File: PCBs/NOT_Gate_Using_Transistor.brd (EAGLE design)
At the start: 23 x 30 mm, 8 parts, among them T1 BC547

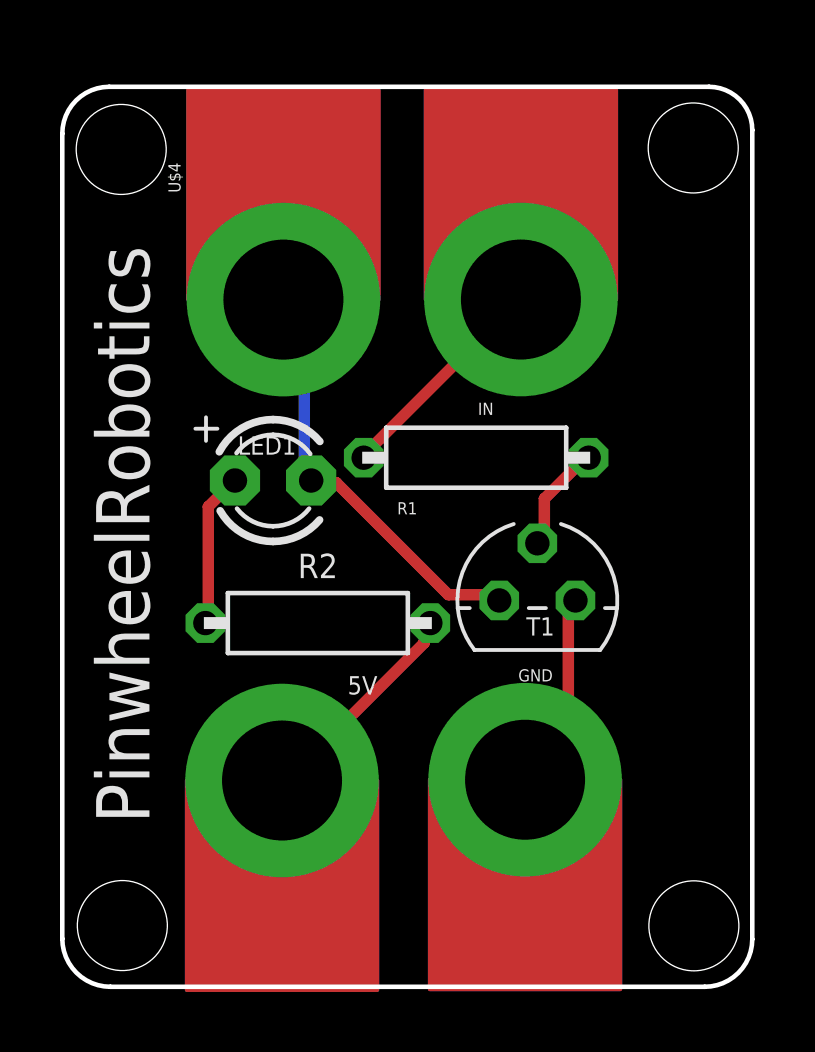
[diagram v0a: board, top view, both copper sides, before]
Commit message: New Update
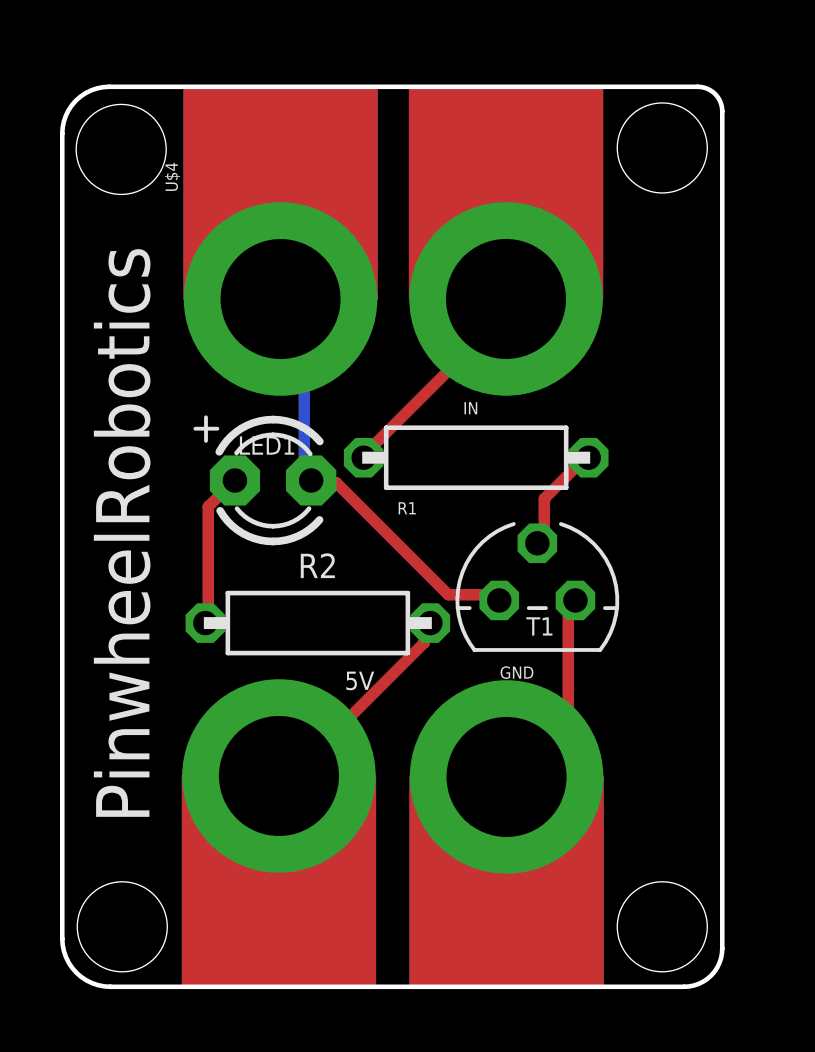
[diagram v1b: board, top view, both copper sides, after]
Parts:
- moved GND 0.62 mm to (11.8, 6.99)
- moved IN 0.50 mm to (11.8, 22.9)
- moved 5V 0.18 mm to (4.22, 7.03)
- moved U$4 0.10 mm to (4.28, 22.9)
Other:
- board size 23 x 30 mm -> 22 x 30 mm
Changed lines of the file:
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@@
 <plain>
 <hole x="-1.036" y="27.912" drill="3"/>
-<hole x="18.031" y="27.961" drill="3"/>
-<hole x="-0.998" y="2.041" drill="3"/>
-<hole x="18.053" y="2.032" drill="3"/>
-<wire x1="-1.3943875" y1="0" x2="18.413571875" y2="0" width="0.1524" layer="20"/>
-<wire x1="18.413571875" y1="0" x2="20" y2="1.586428125" width="0.1524" layer="20" curve="90"/>
-<wire x1="20" y1="1.586428125" x2="20" y2="28.5579125" width="0.1524" layer="20"/>
-<wire x1="20" y1="28.5579125" x2="18.5579125" y2="30" width="0.1524" layer="20" curve="90"/>
-<wire x1="18.5579125" y1="30" x2="-1.437390625" y2="30" width="0.1524" layer="20"/>
+<hole x="17" y="27.961" drill="3"/>
+<hole x="-1" y="2" drill="3"/>
+<hole x="17" y="2" drill="3"/>
+<wire x1="-1.3943875" y1="0" x2="17.7262875" y2="0" width="0.1524" layer="20"/>
+<wire x1="17.7262875" y1="0" x2="19" y2="1.2737125" width="0.1524" layer="20" curve="90"/>
+<wire x1="19" y1="1.2737125" x2="19" y2="29.182434375" width="0.1524" layer="20"/>
+<wire x1="19" y1="29.182434375" x2="18.182434375" y2="30" width="0.1524" layer="20" curve="90"/>
+<wire x1="18.182434375" y1="30" x2="-1.437390625" y2="30" width="0.1524" layer="20"/>
 <wire x1="-1.437390625" y1="30" x2="-3" y2="28.437390625" width="0.1524" layer="20" curve="90"/>
 <wire x1="-3" y1="28.437390625" x2="-3" y2="1.6056125" width="0.1524" layer="20"/>
@@
 </autorouter>
 <elements>
-<element name="5V" library="microbit" package="MICROBIT_PAD" value="MICROBIT_PAD" x="4.325" y="6.876" smashed="yes">
-<attribute name="NAME" x="6.512" y="9.745" size="0.6096" layer="21" font="vector"/>
-</element>
-<element name="GND" library="microbit" package="MICROBIT_PAD" value="MICROBIT_PAD" x="12.426" y="6.902" smashed="yes">
-<attribute name="NAME" x="12.2" y="10.178" size="0.4064" layer="21" font="vector"/>
-</element>
-<element name="IN" library="microbit" package="MICROBIT_PAD" value="MICROBIT_PAD" x="12.288" y="22.909" smashed="yes" rot="R180">
-<attribute name="NAME" x="11.377" y="19.469" size="0.4064" layer="21" font="vector" rot="R180"/>
+<element name="5V" library="microbit" package="MICROBIT_PAD" value="MICROBIT_PAD" x="4.222" y="7.027" smashed="yes">
+<attribute name="NAME" x="6.409" y="9.896" size="0.6096" layer="21" font="vector"/>
+</element>
+<element name="GND" library="microbit" package="MICROBIT_PAD" value="MICROBIT_PAD" x="11.809" y="6.994" smashed="yes">
+<attribute name="NAME" x="11.583" y="10.27" size="0.4064" layer="21" font="vector"/>
+</element>
+<element name="IN" library="microbit" package="MICROBIT_PAD" value="MICROBIT_PAD" x="11.792" y="22.928" smashed="yes" rot="R180">
+<attribute name="NAME" x="10.881" y="19.488" size="0.4064" layer="21" font="vector" rot="R180"/>
 </element>
 <element name="LED1" library="adafruit" library_urn="urn:adsk.eagle:library:420" package="LED3MM" package3d_urn="urn:adsk.eagle:package:6240537/1" value="" x="4.026" y="16.876" smashed="yes">
@@
 <attribute name="VALUE" x="9.694" y="13.628" size="0.6096" layer="27" font="vector" ratio="10" rot="R90"/>
 </element>
-<element name="U$4" library="microbit" package="MICROBIT_PAD" value="MICROBIT_PAD" x="4.371" y="22.906" smashed="yes" rot="R180">
-<attribute name="NAME" x="0.537" y="27.473" size="0.4064" layer="21" font="vector" rot="R270"/>
+<element name="U$4" library="microbit" package="MICROBIT_PAD" value="MICROBIT_PAD" x="4.276" y="22.925" smashed="yes" rot="R180">
+<attribute name="NAME" x="0.442" y="27.492" size="0.4064" layer="21" font="vector" rot="R270"/>
 </element>
 </elements>
@@
 <contactref element="GND" pad="PAD"/>
 <wire x1="13.8684" y1="8.2677" x2="13.8684" y2="12.8016" width="0.381" layer="1"/>
-<wire x1="12.5349" y1="6.9342" x2="13.8684" y2="8.2677" width="0.381" layer="1"/>
+<wire x1="12.92455" y1="7.32385" x2="13.8684" y2="8.2677" width="0.381" layer="1"/>
 <wire x1="13.8684" y1="12.8016" x2="14.106" y2="12.878" width="0.381" layer="1"/>
-<wire x1="12.5349" y1="6.9342" x2="12.426" y2="6.902" width="0.381" layer="1"/>
+<wire x1="12.92455" y1="7.32385" x2="11.809" y2="6.994" width="0.381" layer="1"/>
 </signal>
 <signal name="VOUT">
@@
 <wire x1="5.334" y1="16.8021" x2="5.296" y2="16.876" width="0.381" layer="1"/>
 <wire x1="5.0673" y1="22.1361" x2="5.0673" y2="17.0688" width="0.381" layer="16"/>
-<wire x1="4.5339" y1="22.6695" x2="5.0673" y2="22.1361" width="0.381" layer="16"/>
+<wire x1="4.2837125" y1="22.9196875" x2="5.0673" y2="22.1361" width="0.381" layer="16"/>
 <wire x1="5.0673" y1="17.0688" x2="5.296" y2="16.876" width="0.381" layer="16"/>
-<wire x1="4.5339" y1="22.6695" x2="4.371" y2="22.906" width="0.381" layer="16"/>
+<wire x1="4.2837125" y1="22.9196875" x2="4.276" y2="22.925" width="0.381" layer="16"/>
 </signal>
 <signal name="5V">
@@
 <contactref element="5V" pad="PAD"/>
 <wire x1="9.0678" y1="11.4681" x2="9.0678" y2="12.0015" width="0.381" layer="1"/>
-<wire x1="4.5339" y1="6.9342" x2="9.0678" y2="11.4681" width="0.381" layer="1"/>
+<wire x1="4.78299375" y1="7.18329375" x2="9.0678" y2="11.4681" width="0.381" layer="1"/>
 <wire x1="9.0678" y1="12.0015" x2="9.269" y2="12.124" width="0.381" layer="1"/>
-<wire x1="4.5339" y1="6.9342" x2="4.325" y2="6.876" width="0.381" layer="1"/>
+<wire x1="4.78299375" y1="7.18329375" x2="4.222" y2="7.027" width="0.381" layer="1"/>
 </signal>
 <signal name="N$3">
@@
 <contactref element="IN" pad="PAD"/>
 <contactref element="R1" pad="1"/>
-<wire x1="12.2682" y1="22.9362" x2="7.2009" y2="17.8689" width="0.381" layer="1"/>
+<wire x1="12.06284375" y1="22.73084375" x2="7.2009" y2="17.8689" width="0.381" layer="1"/>
 <wire x1="7.2009" y1="17.8689" x2="7.047" y2="17.636" width="0.381" layer="1"/>
-<wire x1="12.2682" y1="22.9362" x2="12.288" y2="22.909" width="0.381" layer="1"/>
+<wire x1="12.06284375" y1="22.73084375" x2="11.792" y2="22.928" width="0.381" layer="1"/>
 </signal>
 </signals>
